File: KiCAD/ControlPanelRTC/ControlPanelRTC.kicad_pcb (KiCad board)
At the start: 2 copper layers, 50.8 x 63.5 mm, 22 parts, among them J1 Conn_01x04_Pin, J2 Conn_01x04_Pin, Q1 TEPT4400, SW1 SW_Push, SW2 SW_Push, SW3 SW_Push, SW4 SW_Push, U1 DS3231MZ

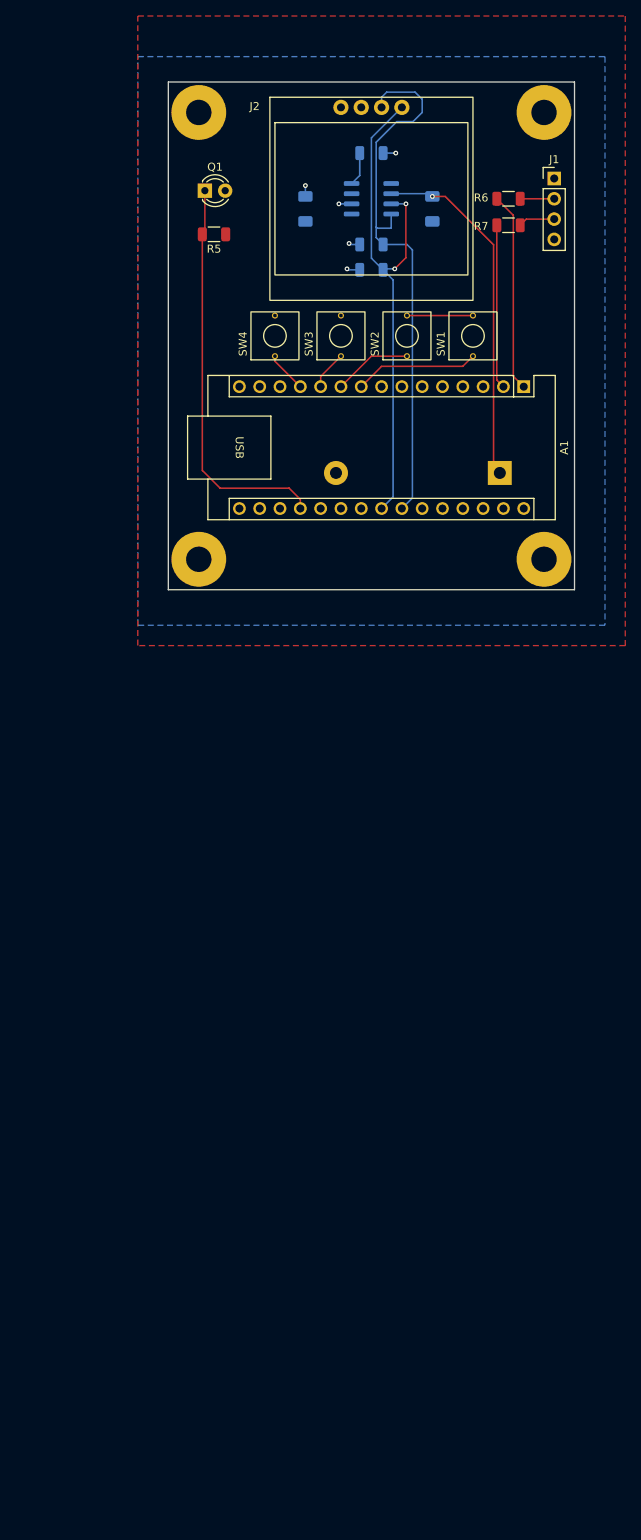
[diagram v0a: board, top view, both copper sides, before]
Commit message: readme
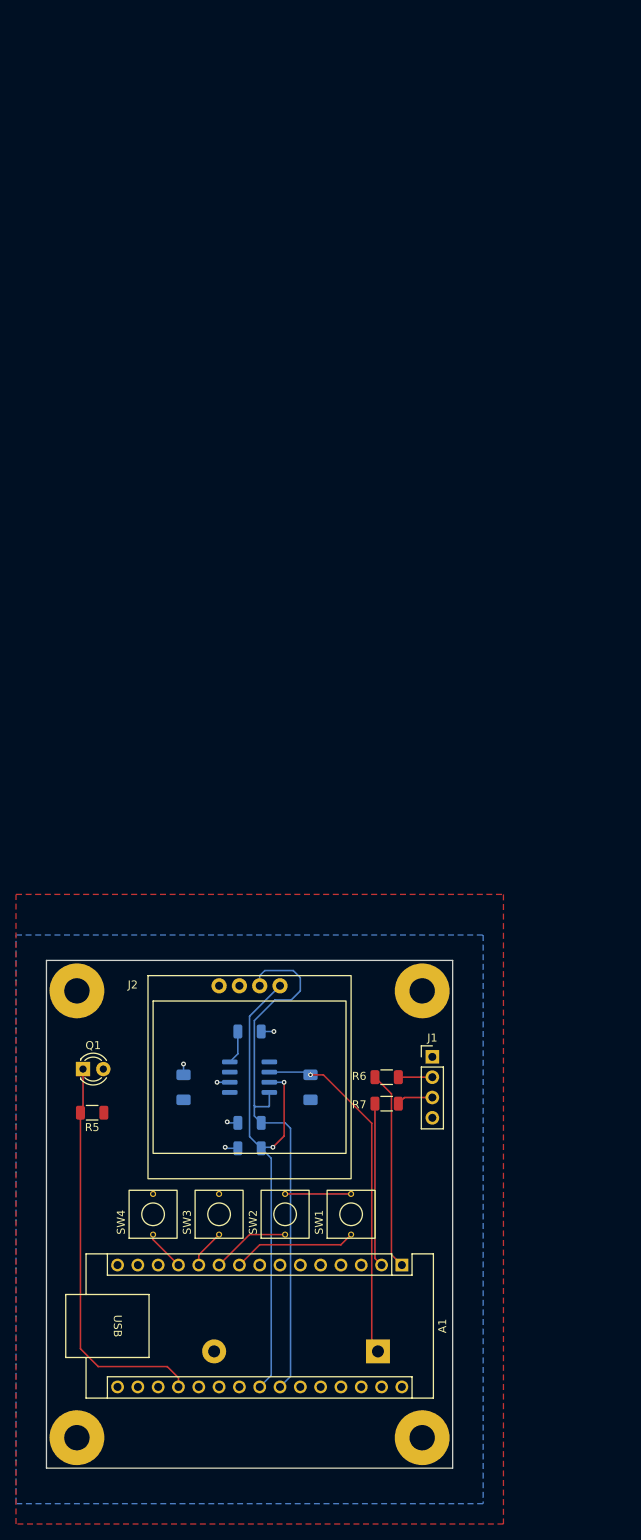
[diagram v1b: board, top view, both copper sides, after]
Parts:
- moved R3 110.9 mm to (128.3, 160.0)
- moved R6 110.9 mm to (145.4, 165.7)
- moved U1 110.9 mm to (128.3, 165.7)
- moved BT1 110.9 mm to (144.3, 200.0)
- moved J2 110.9 mm to (124.5, 154.3)
- moved R2 110.9 mm to (128.3, 174.6)
- moved R5 110.9 mm to (108.6, 170.2)
- moved A1 110.9 mm to (147.3, 189.2)
- moved C1 110.9 mm to (120.0, 167.0)
- moved C2 110.9 mm to (135.9, 167.0)
- moved H1 110.9 mm to (106.7, 154.9)
- moved H2 110.9 mm to (149.9, 154.9)
- moved H3 110.9 mm to (106.7, 210.8)
- moved H4 110.9 mm to (149.9, 210.8)
- moved J1 110.9 mm to (151.1, 163.2)
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
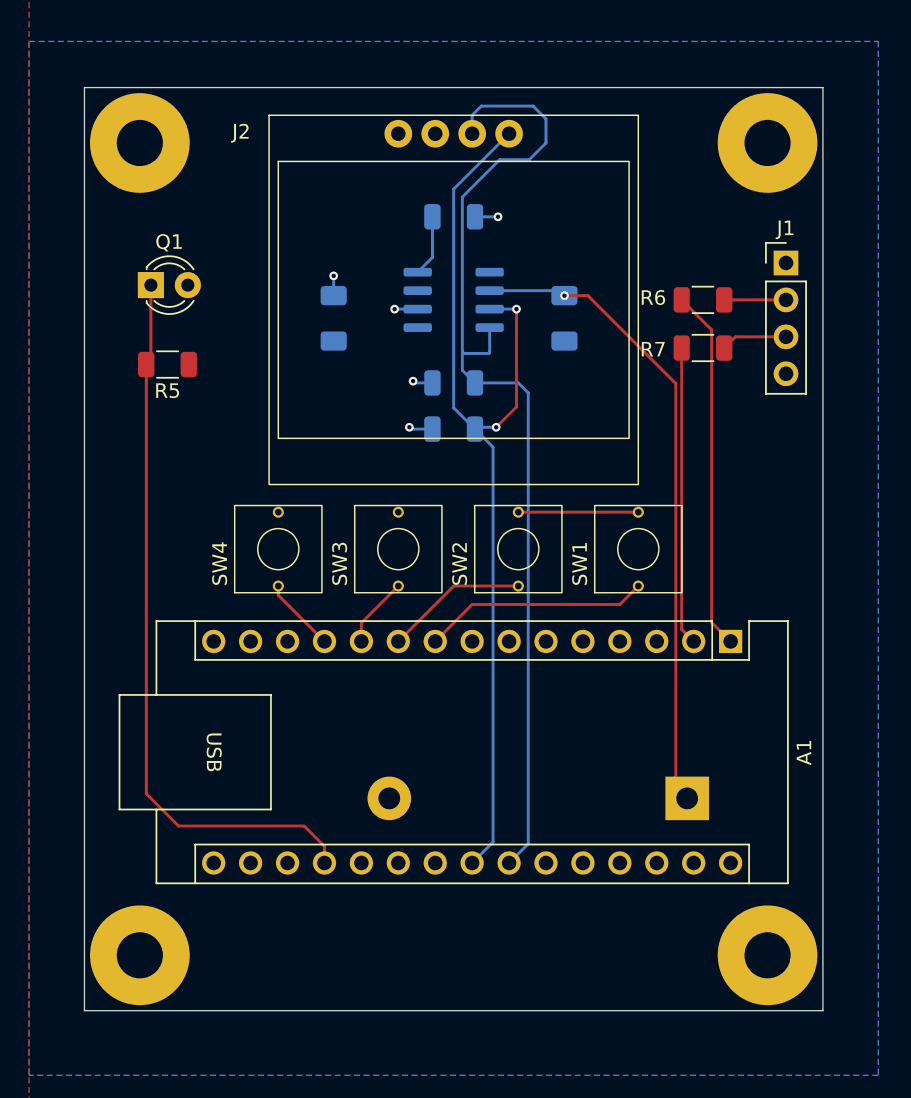
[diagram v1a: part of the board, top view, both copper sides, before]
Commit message: work on control panel
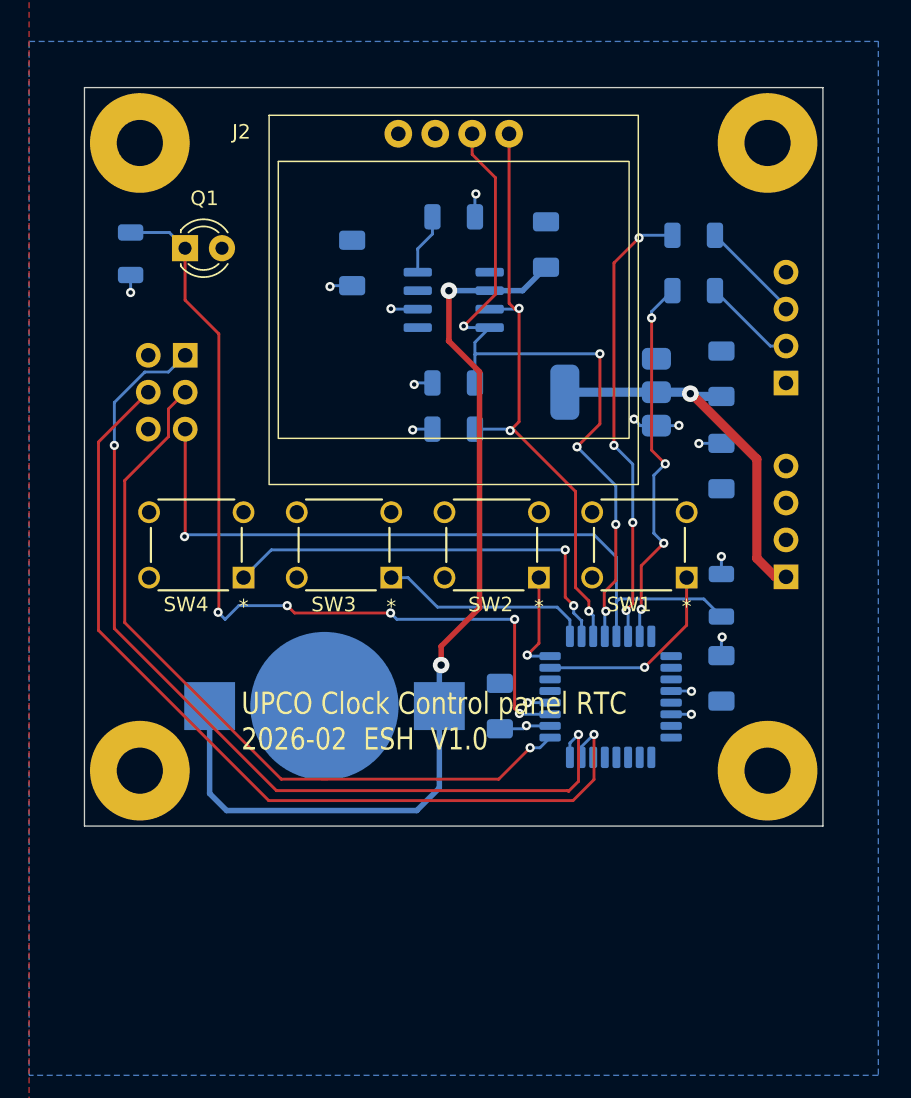
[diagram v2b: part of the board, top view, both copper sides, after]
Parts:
- removed A1: Arduino_Nano_v3.x, Module:Arduino_Nano
- added C3: 10uF, Capacitor_SMD:C_1206_3216Metric_Pad1.33x1.80mm_HandSolder, B.Cu at (146.7, 177.2)
- added C4: 22uF, Capacitor_SMD:C_1206_3216Metric_Pad1.33x1.80mm_HandSolder, B.Cu at (146.7, 170.8)
- added C5: 0.1uF, Capacitor_SMD:C_1206_3216Metric_Pad1.33x1.80mm_HandSolder, B.Cu at (131.4, 193.7)
- added C6: 0.1uF, Capacitor_SMD:C_1206_3216Metric_Pad1.33x1.80mm_HandSolder, B.Cu at (146.7, 191.8)
- added J3: Conn_01x05, Connector_PinHeader_2.54mm:PinHeader_1x04_P2.54mm_Horizontal, B.Cu at (151.1, 184.8)
- added J4: AVR-ISP-6, Connector_PinHeader_2.54mm:PinHeader_2x03_P2.54mm_Horizontal, B.Cu at (109.8, 169.5)
- added R4: 4.7k, Resistor_SMD:R_1206_3216Metric, B.Cu at (146.7, 186.1)
- added U2: AZ1117-3.3, Package_TO_SOT_SMD:SOT-223-3_TabPin2, B.Cu at (139.1, 172.1)
- added U3: ATmega328P-P, Package_QFP:TQFP-32_7x7mm_P0.8mm, B.Cu at (139.1, 193.0)
- BT1: footprint Battery:BatteryHolder_Keystone_103_1x20mm -> Battery:BatteryHolder_Keystone_3000_1x12mm
- J1: value Conn_01x04_Pin -> Conn_01x05; footprint Connector_PinHeader_2.54mm:PinHeader_1x04_P2.54mm_Vertical -> Connector_PinHeader_2.54mm:PinHeader_1x04_P2.54mm_Horizontal; moved to B.Cu
- R1, R2, R3: value R_US -> 4.7k
- R5: moved to B.Cu
- R6, R7: value R_US -> 1k; moved to B.Cu
- SW1, SW2, SW3, SW4: footprint AA_parts:Push_SW -> AA_parts:SW4_1825910-B_TEC
- moved BT1 25.7 mm to (119.4, 193.7)
- moved H3 12.7 mm to (106.7, 198.1)
- moved H4 12.7 mm to (149.9, 198.1)
- moved SW4 9.25 mm to (107.3, 180.3), turned to 180 degrees
- moved J1 8.25 mm to (151.1, 171.4)
- moved R5 8.03 mm to (106.0, 162.6), turned to 90 degrees
- moved R7 7.78 mm to (144.8, 161.3)
- moved SW3 7.43 mm to (117.5, 180.3), turned to 180 degrees
- moved SW2 5.68 mm to (127.6, 180.3), turned to 180 degrees
- moved C2 5.24 mm to (134.6, 161.9), turned to 90 degrees
- moved SW1 4.07 mm to (137.8, 180.3), turned to 180 degrees
- moved C1 4.02 mm to (121.3, 163.2), turned to 90 degrees
- moved Q1 3.46 mm to (109.8, 162.2)
- moved R6 0.90 mm to (144.8, 165.1)
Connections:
- net /ALS renamed /A0
- R6 pad 2: Net-(A1-D1/TX) -> /TXD
- R7 pad 2: Net-(A1-D0/RX) -> /RXD
- SW1 pad 2: GND -> (no net)
- SW2 pad 2: GND -> (no net)
- SW3 pad 2: GND -> (no net)
- SW4 pad 2: GND -> (no net)
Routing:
- net /MISO: track 0.00 -> 63.7 mm, vias 0 -> 2
- net /MOSI: track 0.00 -> 62.4 mm, vias 0 -> 1
- net /SCK: track 0.00 -> 52.5 mm, vias 0 -> 1
- net /~{RESET}: track 0.00 -> 51.1 mm, vias 0 -> 1
- net /RXD: track 0.00 -> 31.5 mm, vias 0 -> 4
- net +3.3V: track 0.00 -> 26.7 mm, vias 0 -> 1
- net /TXD: track 0.00 -> 26.1 mm, vias 0 -> 4
- net Net-(A1-D1/TX): track 24.9 -> 0.00 mm
- net /S3: track 5.13 -> 29.4 mm, vias 0 -> 2
- net /SDA: track 65.5 -> 42.4 mm, vias 2 -> 3
- net +BATT: track 44.3 -> 66.5 mm, vias 1 -> 2
- net Net-(A1-D0/RX): track 20.5 -> 0.00 mm
- net /SCL: track 69.6 -> 51.1 mm, vias 0 -> 5
- net VCC: track 7.56 -> 24.2 mm, vias 5 -> 15
- net /A0: track 50.0 -> 60.3 mm, vias 0 -> 5
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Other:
- board size 50.8 x 63.5 mm -> 50.8 x 50.8 mm
- board text added: "1*"
- board text added: "3.3 -GND- 5V"
- board text added: "ISP"
- board text added: "UPCO Clock Control panel RTC 2026-02 ESH V1.0"
- board text added: "VCC TX RX GND"
